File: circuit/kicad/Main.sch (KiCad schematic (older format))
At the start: 104 parts, among them J1 SH3, J10 PA3, J11 SH4, J2 SH3, J3 FFC6, J4 SH6, J5 FTSH2x5, J6 FFC4, J7 SH4, J8 FFC12, J9 FTSH2x5, Q1 TEMT7100X01, Q10 2N7002T, Q11 TEMT7100X01, Q12 TEMT7100X01, Q13 TEMT7100X01, Q2 TEMT7100X01, Q3 TEMT7100X01, Q4 TEMT7100X01, Q5 TEMT7100X01, Q6 TEMT7100X01, Q7 TEMT7100X01, Q8 TEMT7100X01, Q9 TEMT7100X01, SW1 SKRPABE010, U1 ASTMLPA-16MHz-LJ-E-T, U2 STM32F405RGTx, U3 ICM-20648

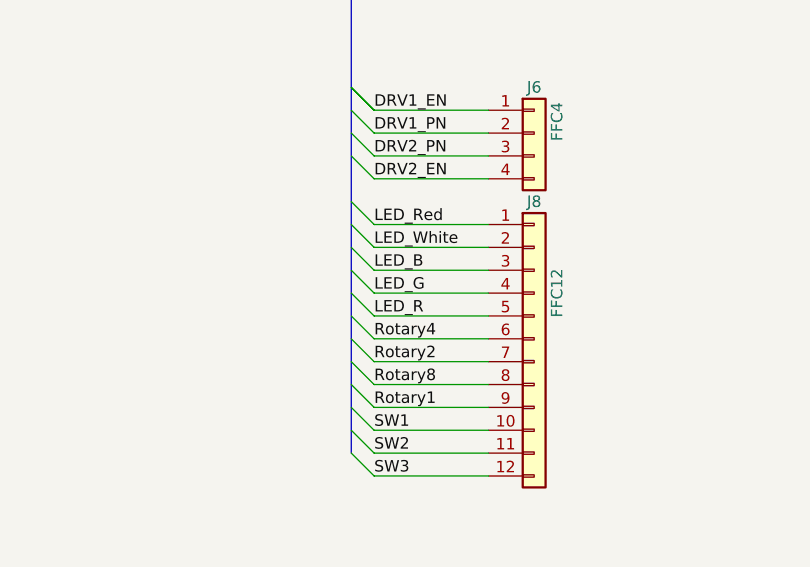
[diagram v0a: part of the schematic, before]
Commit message: hoge
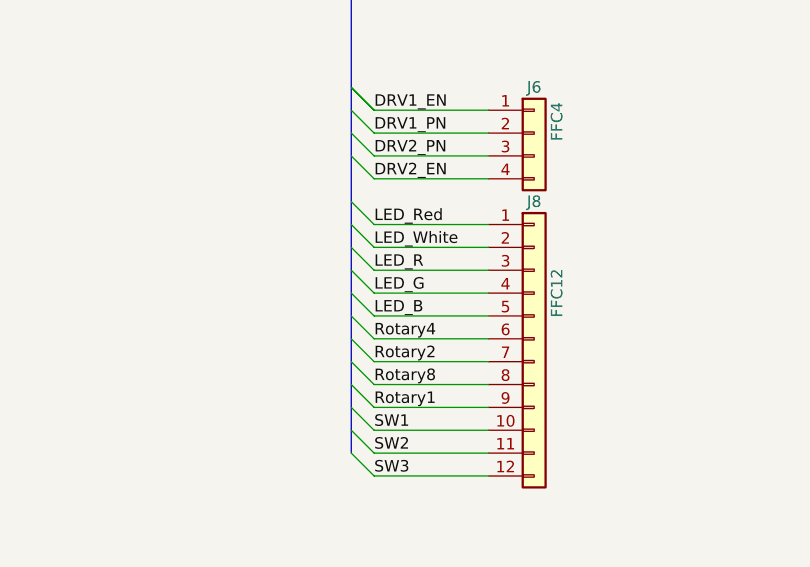
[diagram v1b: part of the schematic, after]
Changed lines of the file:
@@
 Text Label 9000 13300 0    50   ~ 0
 Rotary8
-Text Label 9000 13000 0    50   ~ 0
+Text Label 9000 12800 0    50   ~ 0
 LED_R
 Text Label 9000 12900 0    50   ~ 0
 LED_G
-Text Label 9000 12800 0    50   ~ 0
+Text Label 9000 13000 0    50   ~ 0
 LED_B
 Entry Wire Line
@@
 Wire Wire Line
 	7650 7350 9050 7350
+Text Notes 15050 2000 0    50   ~ 0
+20mA
+Text Notes 18100 1500 0    50   ~ 0
+All : 480mA
+Text Notes 12650 6250 0    50   ~ 0
+All:72mA
+Text Notes 6150 12400 0    50   ~ 0
+5V : under 100mA\n3.3V : under 600mA
 Wire Bus Line
 	19750 5950 19750 8850
@@
 Wire Bus Line
 	8900 11200 8900 13600
-Text Notes 15050 2000 0    50   ~ 0
-20mA
-Text Notes 18100 1500 0    50   ~ 0
-All : 480mA
-Text Notes 12650 6250 0    50   ~ 0
-All:72mA
-Text Notes 6150 12400 0    50   ~ 0
-5V : under 100mA\n3.3V : under 600mA
 $EndSCHEMATC
